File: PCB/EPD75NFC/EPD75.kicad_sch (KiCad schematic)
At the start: 151 parts, among them J1 Conn_01x26, J10 TF_PUSH, J11 Reset, J12 TC2030-USB-NL-DS, J2 PWR, J3 NFC, J4 BTN, J5 USB-C-Socket-H, J7 USB-C-Socket-H, J8 PWR, Q1 BSS138, SW2 ESE13V01D, U2 PN532, U3 MD8942, U4 ESP32-S3-MINI-1, Y1 27.12MHz

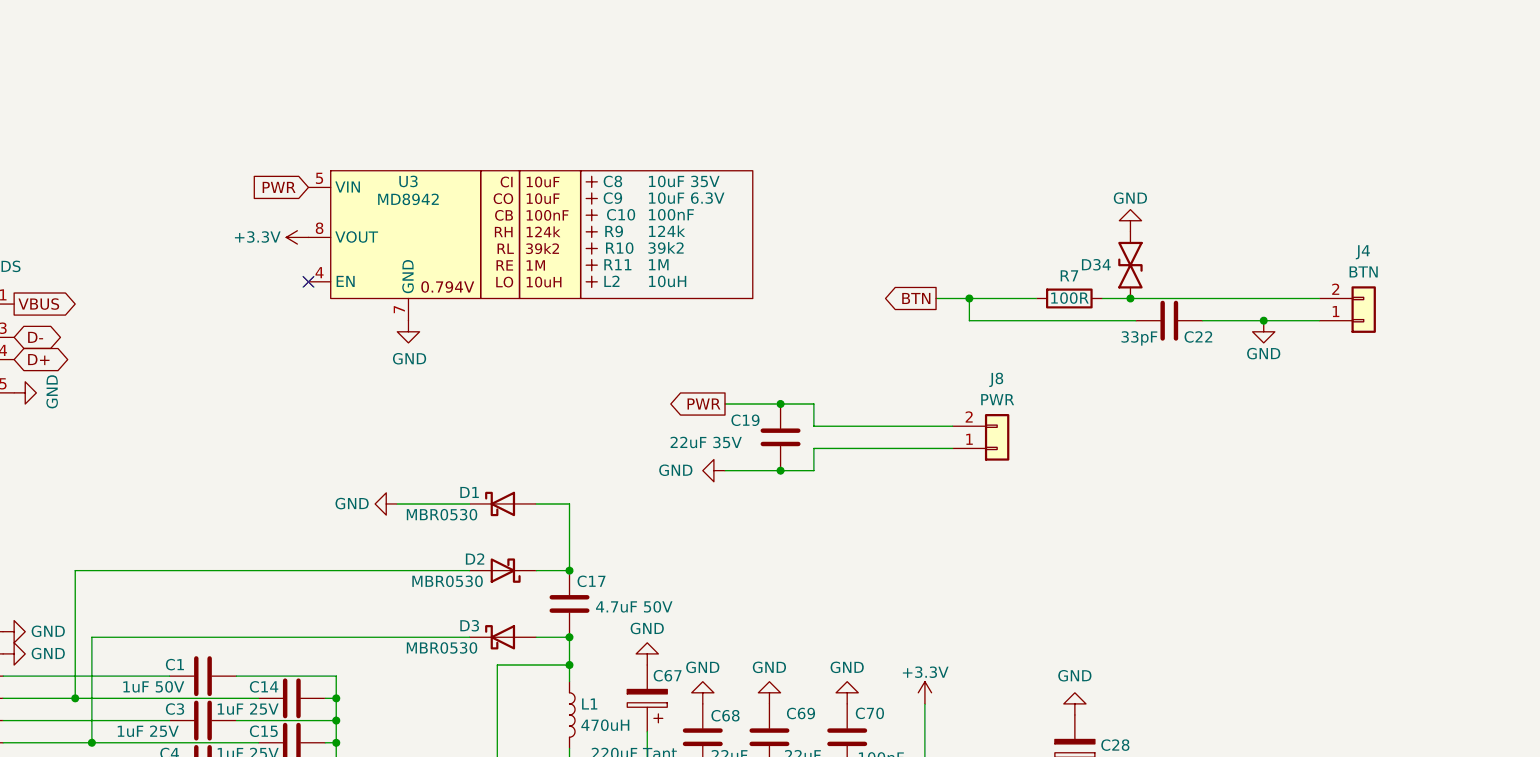
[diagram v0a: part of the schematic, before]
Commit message: Regulator update
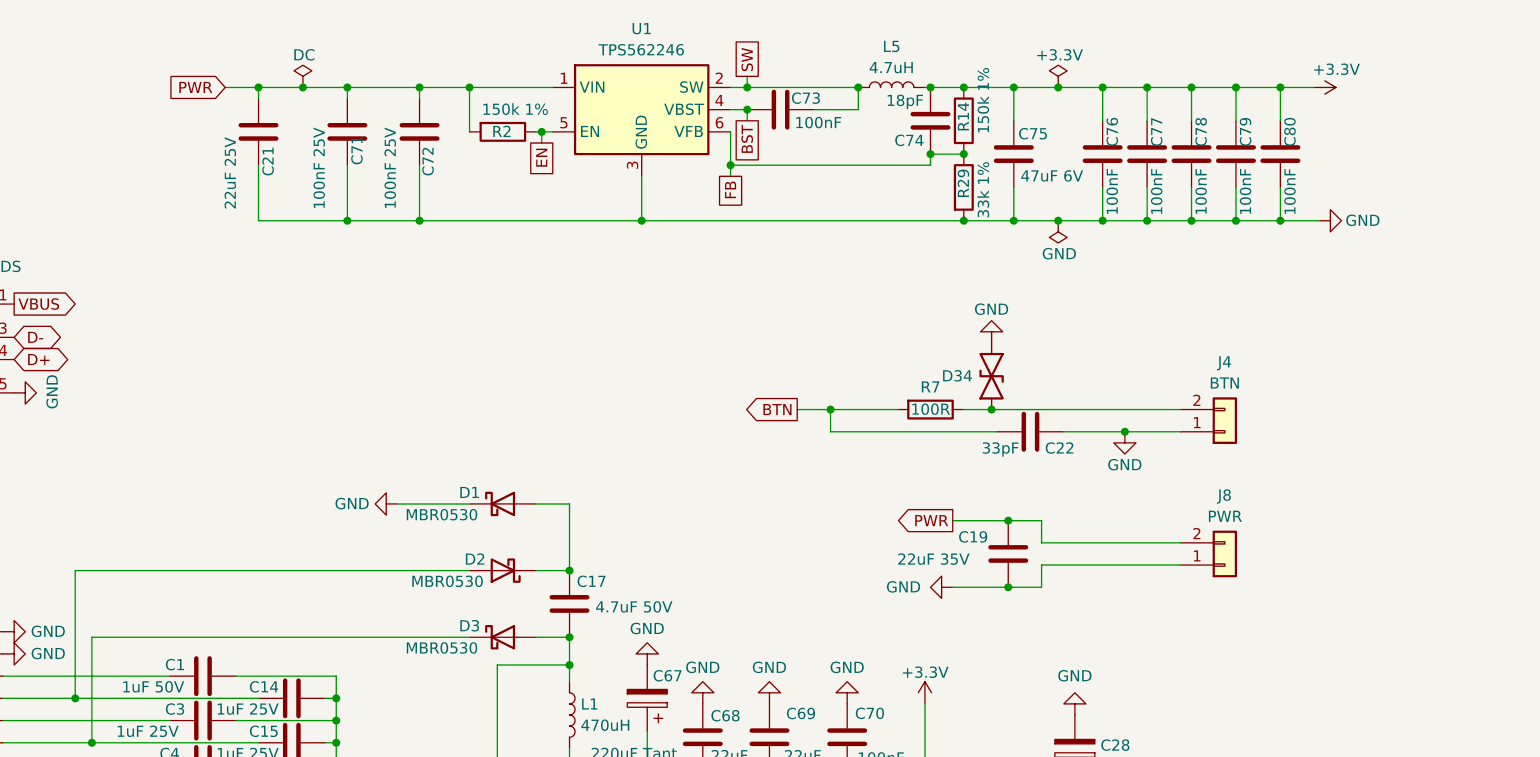
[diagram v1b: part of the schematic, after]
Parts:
- removed C10: 100nF, RevK:C_0603_, symbol RevK:Hidden
- removed C8: 10uF 35V, RevK:C_0603_, symbol RevK:Hidden
- removed C9: 10uF 6.3V, RevK:C_0603_, symbol RevK:Hidden
- removed L2: 10uH, RevK:L_4x4_, symbol RevK:Hidden
- removed R10: 39k2, RevK:R_0402_, symbol RevK:Hidden
- removed R11: 1M, RevK:R_0402_, symbol RevK:Hidden
- removed R9: 124k, RevK:R_0402_, symbol RevK:Hidden
- removed U3: MD8942, RevK:SOT-23-6-MD8942, symbol RevK:MD89420-RegBlock
- added C21: 22uF 25V, RevK:C_0805, symbol Device:C
- added C71, C72: 100nF 25V, RevK:C_0402, symbol Device:C
- added C73, C76, C77, C78, C79, C80: 100nF, RevK:C_0201, symbol Device:C
- added C74: 18pF, RevK:C_0201, symbol Device:C
- added C75: 47uF 6V, RevK:C_0805, symbol Device:C
- added L5: 4.7uH, RevK:L_5x5, symbol Device:L
- added R14, R2: 150k 1%, RevK:R_0201, symbol Device:R
- added R29: 33k 1%, RevK:R_0201, symbol Device:R
- added U1: TPS562246, RevK:SOT-563, symbol RevK:TPS562246
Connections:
- net +3.3V: now also C74.2, C75.1, C76.2, C77.2, C78.2, C79.2, C80.2, L5.2, R14.1
- net GND: now also C21.2, C71.2, C72.2, C75.2, C76.1, C77.1, C78.1, C79.1, C80.1, R29.2, U1.3 (GND)
- net PWR: now also C21.1, C71.1, C72.1, R2.2, U1.1 (VIN)
- new net BST: C73.1, U1.4 (VBST)
- new net EN: R2.1, U1.5 (EN)
- new net FB: C74.1, R14.2, R29.1, U1.6 (VFB)
- new net SW: C73.2, L5.1, U1.2 (SW)
- no-connect marks 41 -> 40
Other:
- moved on the sheet: C19, C22, D34, J4, J8, R7

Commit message: Library update
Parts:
- L1: footprint RevK:L_4x4 -> RevK:L_6x6; MPN C42429207 -> C168100
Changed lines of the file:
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@@
 			)
 		)
-		(property "Footprint" "RevK:L_4x4"
+		(property "Footprint" "RevK:L_6x6"
 			(at 187.96 93.98 0)
 			(effects
@@
 			)
 		)
-		(property "MPN" "C42429207"
+		(property "MPN" "C168100"
 			(at 187.96 93.98 0)
 			(effects

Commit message: Library update
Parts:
- added C8, C81, C83, C9: 100nF, RevK:C_0201, symbol Device:C
- added T1: T3902_MEMS_Mic, RevK:T3902_MEMS_Mic_Open, symbol RevK:T3902_MEMS_Mic
- added U3: SCD41, RevK:SCD41, symbol RevK:SCD41
- added U5: GZP6816D, RevK:Bosch_LGA-8_2x2.5mm_P0.65mm_ClockwisePinNumbering, symbol RevK:GZP6816D
- added U7: SHT40, RevK:Sensirion_DFN-4_1.5x1.5mm_P0.5mm_SHT4x-Side, symbol RevK:SHT40
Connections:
- net +3.3V: now also C8.2, C81.2, C83.2, C9.2, T1.2 (SELECT), T1.5 (VDD), U3.19 (VDDH), U3.7 (VDD), U5.8 (VDD), U7.3 (VDD)
- net GND: now also C8.1, C81.1, C83.1, C9.1, T1.3 (GND), U3.20 (GND), U3.21 (GND), U3.6 (GND), U5.1 (GND), U5.7 (GND), U7.4 (VSS)
- net SCL: now reaches U4.19 (GPIO15)
- net SCL: now also U3.9 (SCL), U5.4 (SCL), U7.2 (SCL)
- net SDA: now reaches U4.20 (GPIO16)
- net SDA: now also U3.10 (SDA), U5.3 (SDA), U7.1 (SDA)
- net MDATA: now reaches U4.21 (GPIO17)
- net MDATA: now also T1.1 (DATA)
- net MCLK: now reaches U4.22 (GPIO18)
- net MCLK: now also T1.4 (CLK)
- no-connect marks 40 -> 36
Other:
- note added: "Left"
- moved on the sheet: A1, C35, C42, C49, C50, C51, C52, C53, C54, C55, C56, C57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
